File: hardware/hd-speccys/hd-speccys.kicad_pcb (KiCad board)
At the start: 2 copper layers, 68.6 x 68.6 mm, 52 parts, among them J1 POWER 9-20VDC, J2 PI_ZERO, J3 ULA_SOCKET, J4 ULA_ZX, J5 UART, J6 Debug_Data, J7 Debug_Ctrl, J8 GND, U1 74LS541, U2 74LS541, U3 74LS10, U4 TSR_1-2450, U5 74AHC1G32

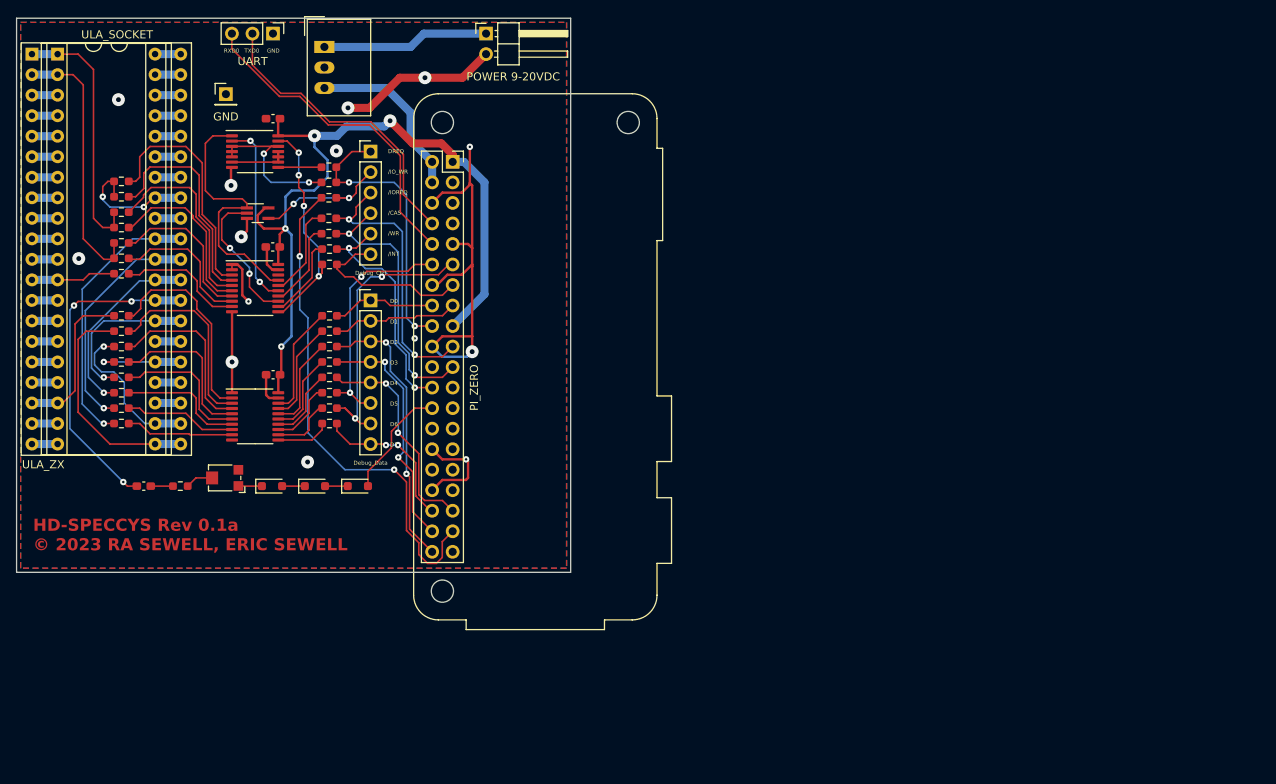
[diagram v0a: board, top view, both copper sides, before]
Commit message: hw: board updates
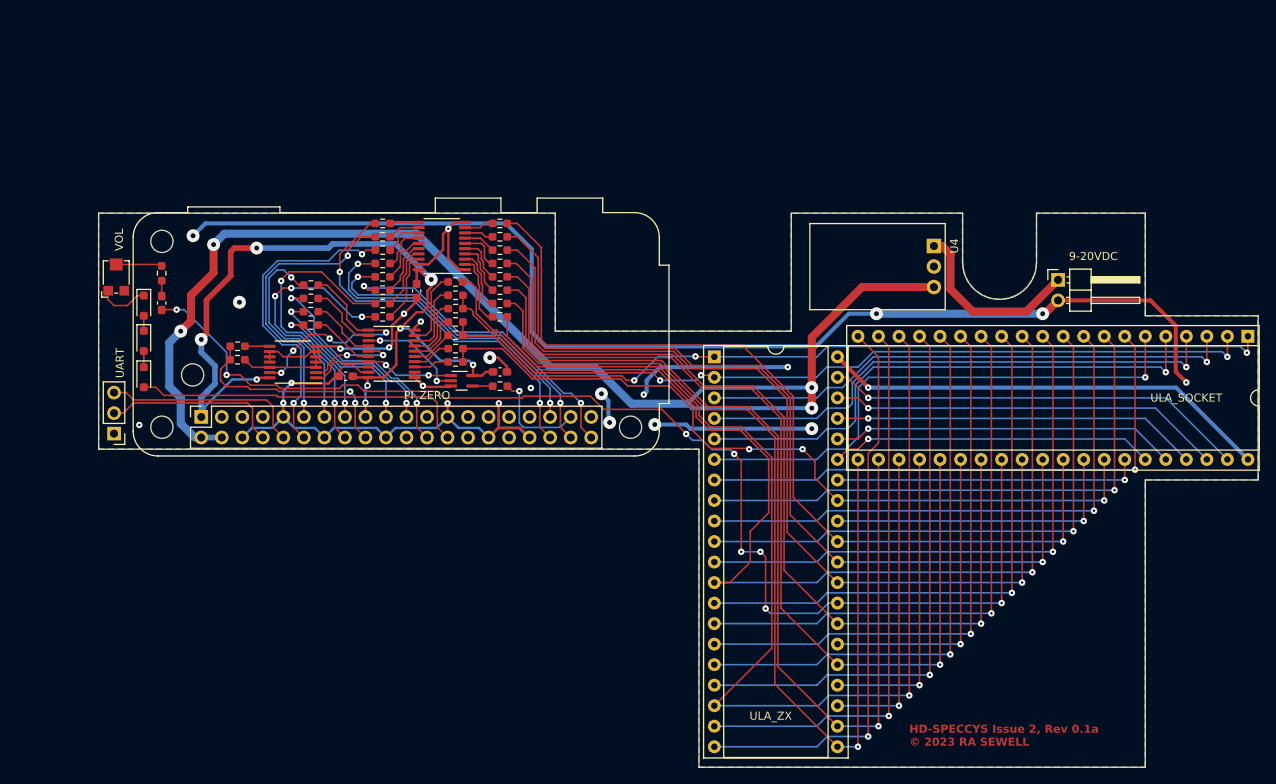
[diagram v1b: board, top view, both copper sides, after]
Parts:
- removed J6: Debug_Data, Connector_PinHeader_2.54mm:PinHeader_1x08_P2.54mm_Vertical
- removed J7: Debug_Ctrl, Connector_PinHeader_2.54mm:PinHeader_1x06_P2.54mm_Vertical
- removed J8: GND, Connector_PinHeader_2.54mm:PinHeader_1x01_P2.54mm_Vertical
- added ?: , , F.Cu at (85.3, 82.2)
- J1: value POWER 9-20VDC -> 9-20VDC
- U4: footprint Converter_DCDC:Converter_DCDC_TRACO_TSR-1_THT -> Converter_DCDC:Converter_DCDC_Murata_OKI-78SR_Horizontal
- moved J3 151.4 mm to (215.9, 77.5), turned to -90 degrees
- moved J4 92.4 mm to (149.9, 80.0)
- moved U4 79.4 mm to (177.0, 66.3)
- moved J1 77.1 mm to (192.4, 70.5)
- moved J5 53.3 mm to (75.6, 89.5), turned to 180 degrees
- moved R16 53.0 mm to (123.3, 63.5), turned to 0 degrees
- moved R15 51.4 mm to (123.3, 65.2), turned to 0 degrees
- moved R14 50.1 mm to (123.3, 66.8), turned to 0 degrees
- moved R13 48.9 mm to (123.3, 68.5), turned to 0 degrees
- moved R12 48.0 mm to (123.3, 70.1), turned to 0 degrees
- moved R11 47.4 mm to (123.3, 71.8), turned to 0 degrees
- moved R2 47.0 mm to (117.8, 80.6), turned to 0 degrees
- moved R10 47.0 mm to (123.3, 73.4), turned to 0 degrees
- moved R9 46.8 mm to (123.3, 75.1), turned to 0 degrees
- moved R3 45.4 mm to (117.8, 79.0), turned to 0 degrees
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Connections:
- J2 pad 31: unconnected-(J2-SOE_SE-Pad31) -> Net-(J2-SOE_SE)
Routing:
- net GND: track 116.0 -> 359.6 mm, vias 14 -> 25
- net VDD: track 21.8 -> 157.0 mm, vias 0 -> 4
- net Net-(J3-/INT): track 10.5 -> 138.3 mm, vias 0 -> 1
- net Net-(J3-D0): track 19.5 -> 145.3 mm, vias 0 -> 1
- net Net-(J3-MIC_TAPE): track 40.1 -> 150.4 mm, vias 3 -> 8
- net Net-(J3-D3): track 10.8 -> 116.7 mm
- net Net-(J3-D2): track 19.4 -> 121.6 mm
- net Net-(J3-D1): track 28.2 -> 122.3 mm, vias 0 -> 1
- net Net-(J3-D4): track 19.3 -> 113.2 mm
- net Net-(J3-D5): track 23.7 -> 111.1 mm
- net Net-(J3-D6): track 28.8 -> 110.2 mm
- net Net-(J3-/IOREQ): track 15.7 -> 96.6 mm, vias 2 -> 3
- net Net-(J3-D7): track 33.9 -> 109.3 mm
- net Net-(J3-/CAS): track 31.7 -> 105.2 mm, vias 0 -> 3
- net Net-(J3-/WR): track 32.7 -> 104.7 mm, vias 0 -> 3
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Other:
- board size 68.6 x 68.6 mm -> 143.5 x 68.6 mm
- board text added: "HD-SPECCYS Issue 2, Rev 0.1a © 2023 RA SEWELL"
- board text added: "VOL"
- board text removed: "/CAS"
- board text removed: "/INT"
- board text removed: "/IOREQ"
- board text removed: "/IO_WR"
- board text removed: "/WR"
- board text removed: "D0"
- board text removed: "D1"
- board text removed: "D2"
- board text removed: "D3"
- board text removed: "D4"
- board text removed: "D5"
- board text removed: "D6"
- board text removed: "D7"
- board text removed: "DREQ"
- board text removed: "GND"
- board text removed: "HD-SPECCYS Rev 0.1a © 2023 RA SEWELL, ERIC SEWELL"
- board text removed: "RXD0"
- board text removed: "TXD0"
